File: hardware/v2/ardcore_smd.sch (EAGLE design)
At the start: 96 parts, among them IC1 OPA2171, IC11 74AHCT1G125DBV, IC12 LM4040B25, IC2 7805DT, IC3 OPA2171, IC5 74AHCT1G125DBV, IC6 ATMEGA328P-AU, IC7 74AHCT1G125DBV, IC8 74AHCT1G125DBV, IC9 LM4040B10, U2 DAC8552IDGKT, Y1 RESONATORSMD

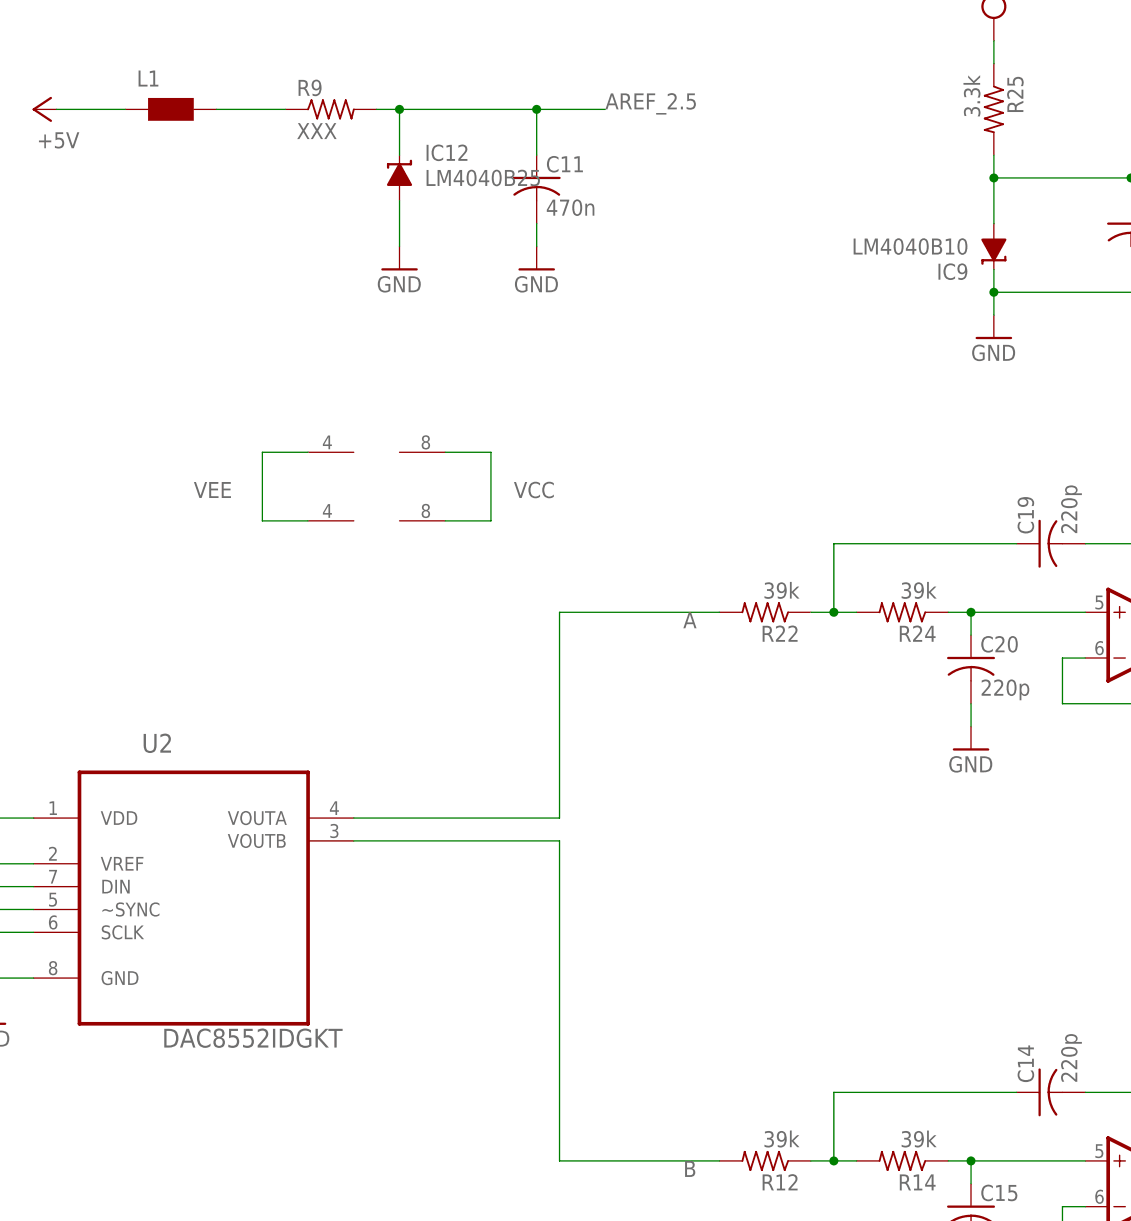
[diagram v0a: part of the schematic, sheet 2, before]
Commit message: Adding version
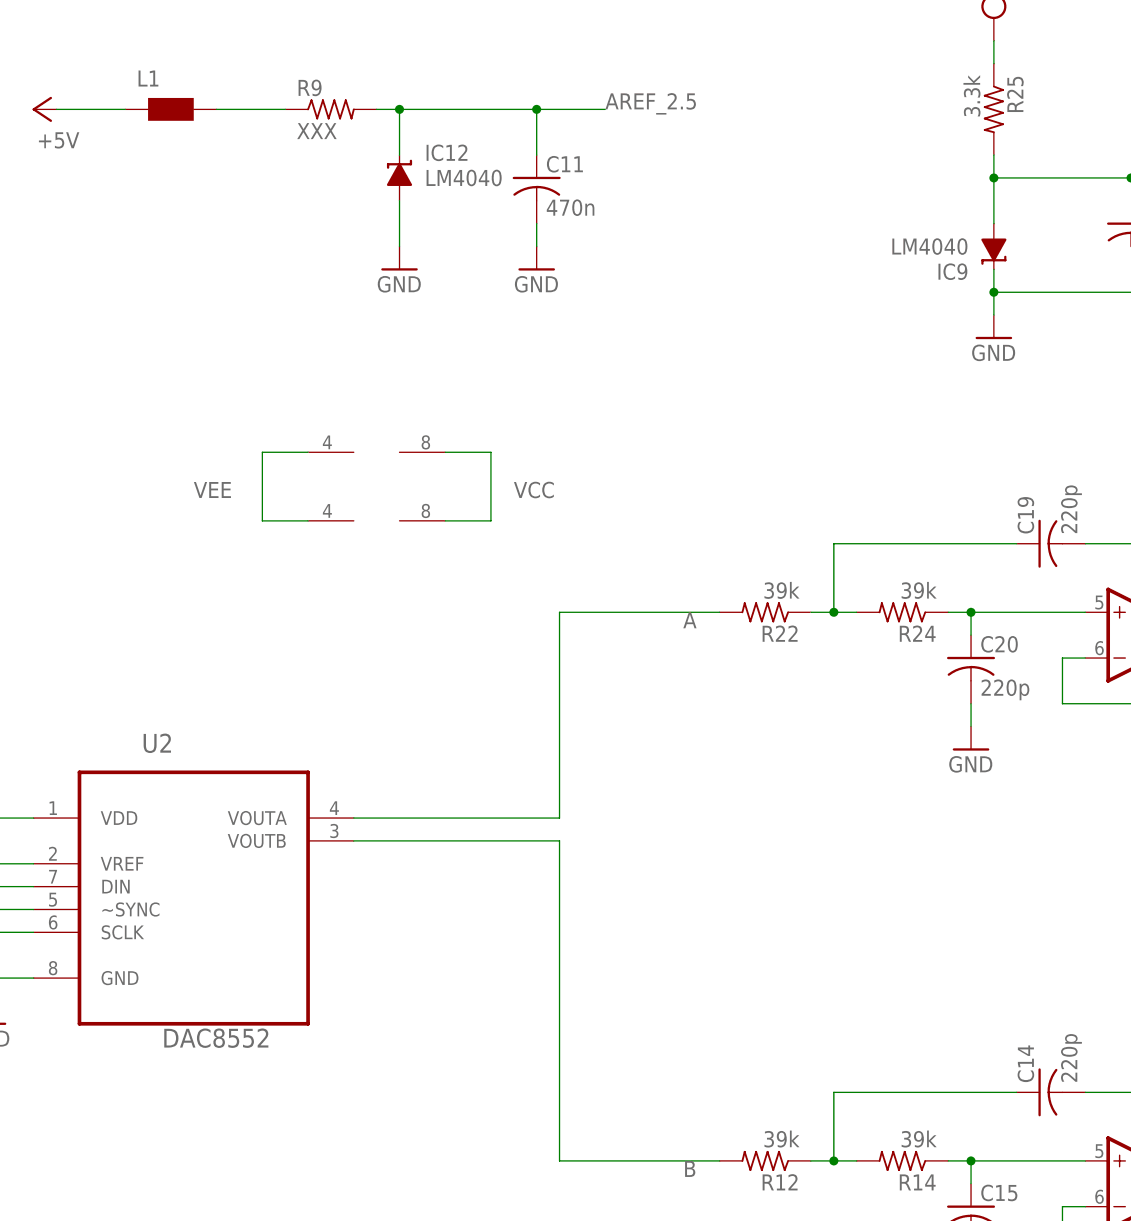
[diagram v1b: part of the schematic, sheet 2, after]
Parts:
- IC12: value LM4040B25 -> LM4040
- IC9: value LM4040B10 -> LM4040
- U2: value DAC8552IDGKT -> DAC8552
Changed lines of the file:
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@@
 <?xml version="1.0" encoding="utf-8"?>
 <!DOCTYPE eagle SYSTEM "eagle.dtd">
-<eagle version="7.3.0">
+<eagle version="7.6.0">
 <drawing>
 <settings>
@@
 <part name="D7" library="hhn_diodes_smd" deviceset="LL4148" device=""/>
 <part name="D8" library="hhn_diodes_smd" deviceset="LL4148" device=""/>
-<part name="U2" library="Texas Instruments_By_element14_Batch_1" deviceset="DAC8552IDGKT" device=""/>
+<part name="U2" library="Texas Instruments_By_element14_Batch_1" deviceset="DAC8552IDGKT" device="" value="DAC8552"/>
 <part name="IC1" library="linear" deviceset="TL072" device="D" value="OPA2171"/>
 <part name="R12" library="rcl" deviceset="R-US_" device="R0603" value="39k"/>
@@
 <part name="GND14" library="SparkFun" deviceset="GND" device=""/>
 <part name="L1" library="wuerth-elektronik" deviceset="WE-CBF" device="_0603"/>
-<part name="IC9" library="texas" deviceset="LM4041" device="DBZ" technology="B12" value="LM4040B10"/>
+<part name="IC9" library="texas" deviceset="LM4041" device="DBZ" technology="B12" value="LM4040"/>
 <part name="R25" library="rcl" deviceset="R-US_" device="R0603" value="3.3k"/>
 <part name="C22" library="rcl" deviceset="C-US" device="C0603" value="470n"/>
 <part name="GND69" library="SparkFun" deviceset="GND" device=""/>
 <part name="SUPPLY3" library="supply2" deviceset="VEE" device=""/>
-<part name="IC12" library="texas" deviceset="LM4041" device="DBZ" technology="B12" value="LM4040B25"/>
+<part name="IC12" library="texas" deviceset="LM4041" device="DBZ" technology="B12" value="LM4040"/>
 <part name="R9" library="rcl" deviceset="R-US_" device="R0603" value="XXX"/>
 <part name="GND24" library="SparkFun" deviceset="GND" device=""/>
